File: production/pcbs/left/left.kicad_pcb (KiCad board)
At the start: 2 copper layers, 90 x 71 mm, 43 parts, among them T1 Flactyl 4.2 (left)

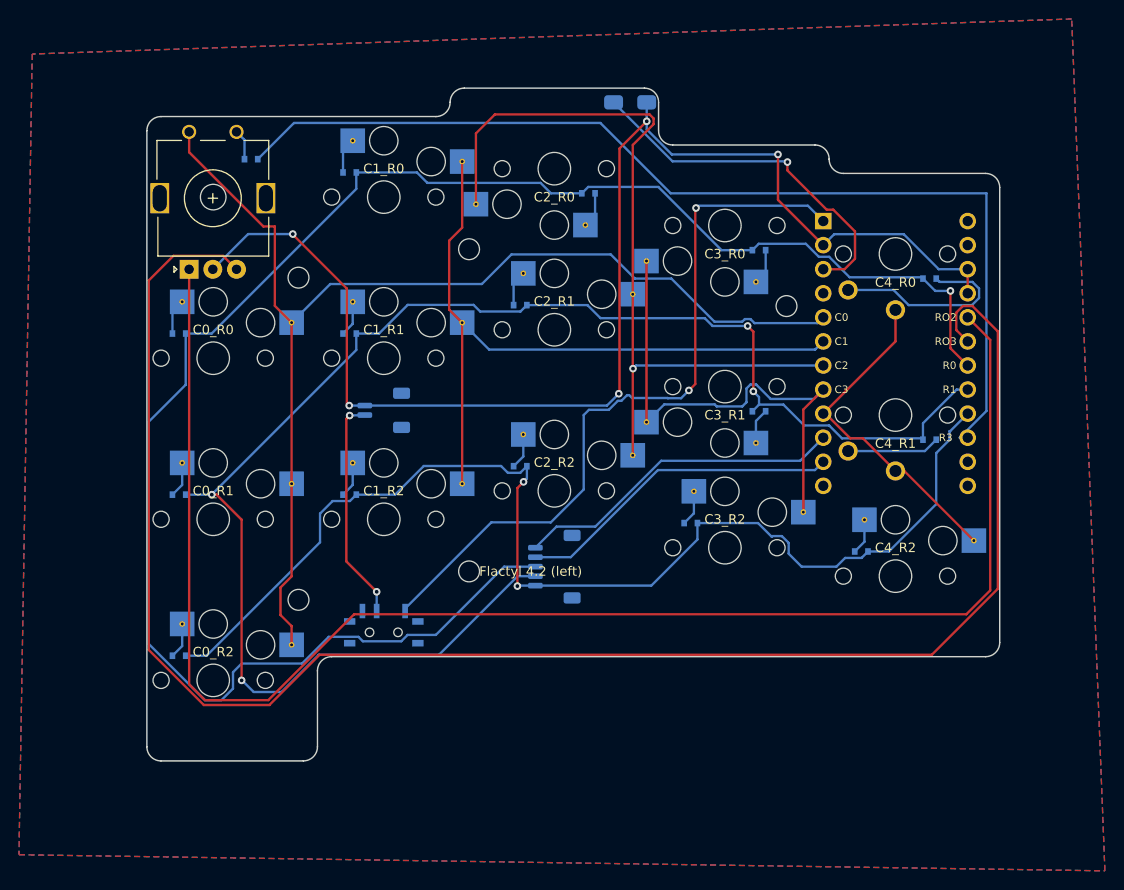
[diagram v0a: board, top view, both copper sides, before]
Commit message: Update pcb to 4.2
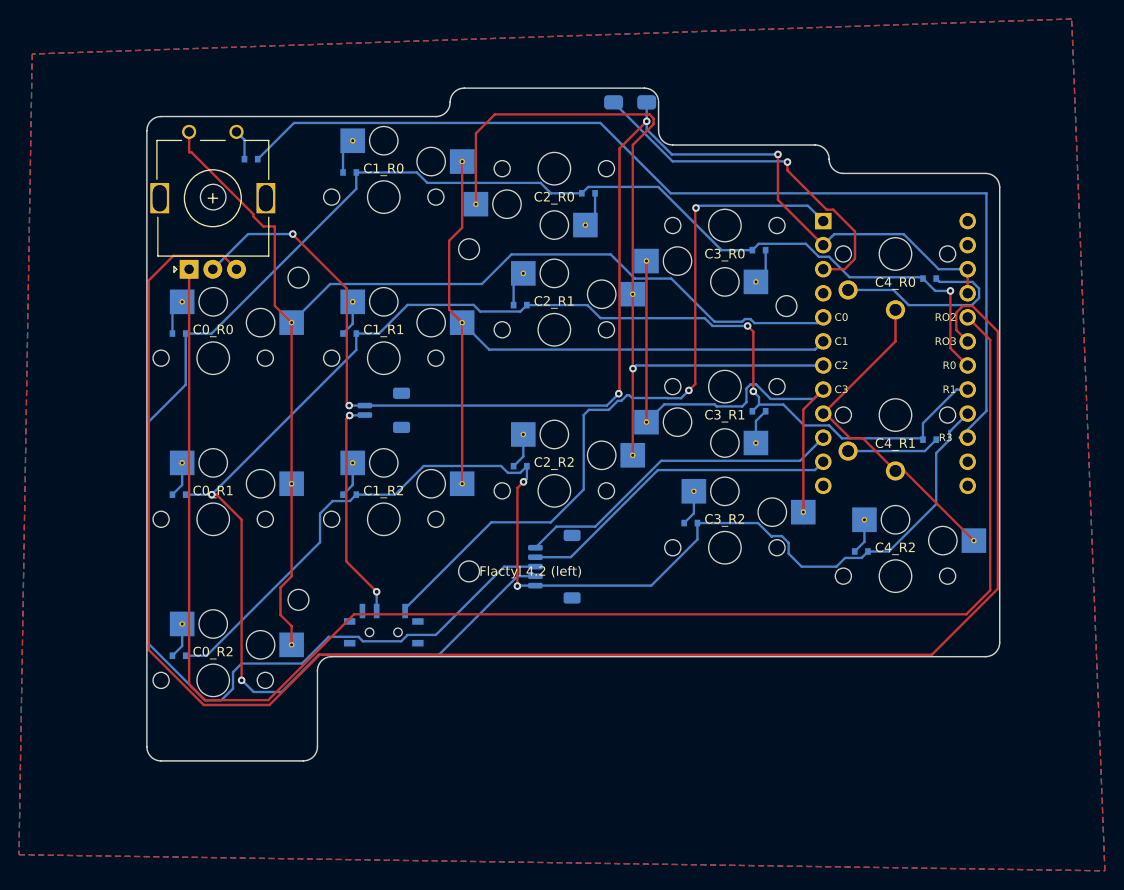
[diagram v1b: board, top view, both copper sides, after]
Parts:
- T1: moved to F.Cu
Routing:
- net C4_R0: track 188.5 -> 0.00 mm, vias 1 -> 0
- net R0: track 3.77 -> 188.5 mm, vias 0 -> 1
- net P0: track 183.5 -> 0.00 mm
- net P3: track 3.77 -> 183.5 mm
- net P1: track 163.6 -> 0.00 mm
- net P2: track 3.77 -> 163.6 mm
- net C4_R1D: track 164.4 -> 9.80 mm, vias 4 -> 0
- net P8: track 109.4 -> 0.00 mm
- net R3: track 3.77 -> 109.4 mm
- net C4: track 122.9 -> 35.6 mm
- net P9: track 77.8 -> 0.00 mm, vias 2 -> 0
- net RAW: track 3.77 -> 77.8 mm, vias 0 -> 2
- net C1: track 3.77 -> 74.8 mm
- net GND: track 83.9 -> 138.6 mm, vias 1 -> 5
- net three: track 53.2 -> 0.00 mm
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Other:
- net class Default removed
